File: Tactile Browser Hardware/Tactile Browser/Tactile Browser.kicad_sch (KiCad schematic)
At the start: 78 parts, among them SW1 SW_Push, SW10 SW_Push, SW11 SW_Push, SW12 SW_Push, SW13 SW_Push, SW14 SW_Push, SW15 SW_Push, SW16 SW_Push, SW17 SW_Push, SW18 SW_Push, SW19 SW_Push, SW2 SW_Push, SW20 SW_Push, SW3 SW_Push, SW4 SW_Push, SW5 SW_Push, SW6 SW_Push, SW7 SW_Push, SW8 SW_Push, SW9 SW_Push

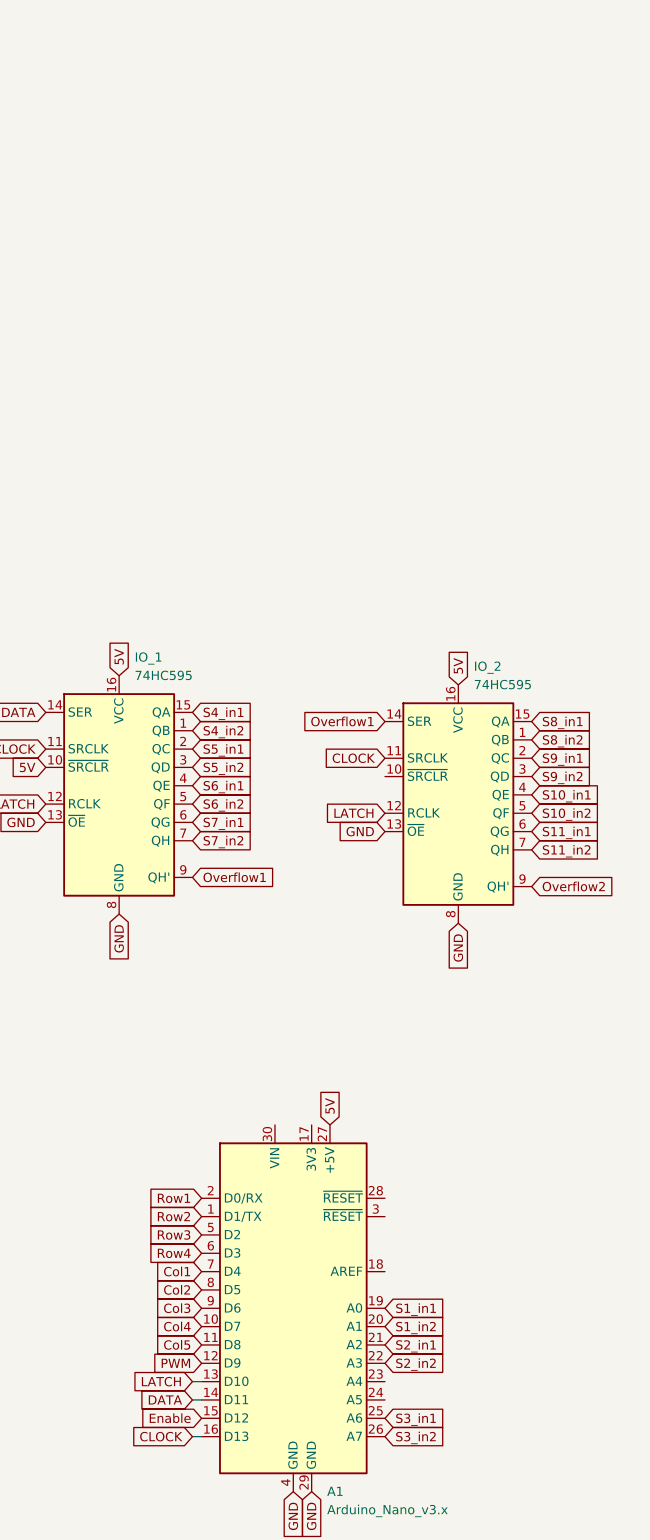
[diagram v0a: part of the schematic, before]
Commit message: I2C
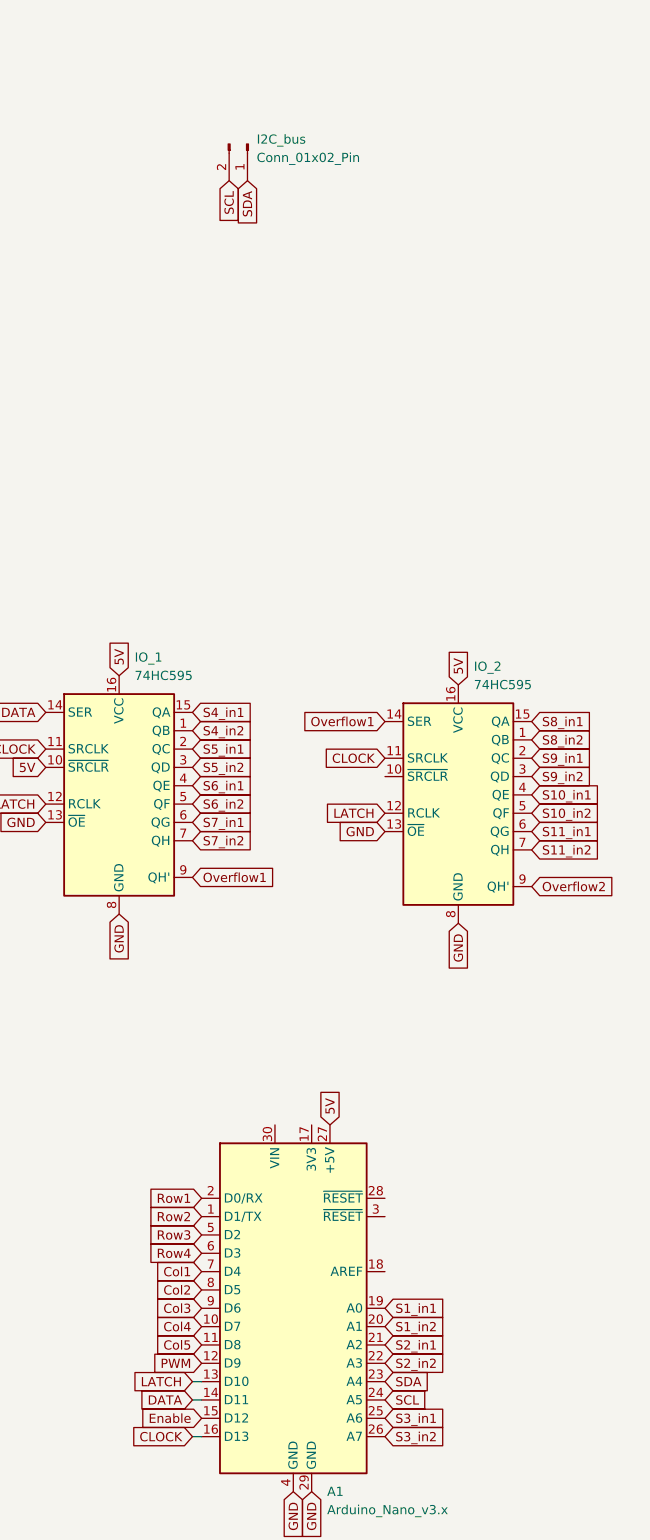
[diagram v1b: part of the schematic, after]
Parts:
- added I2C_bus: Conn_01x02_Pin, symbol Connector:Conn_01x02_Pin
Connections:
- net SDA: now reaches A1.23 (A4)
- net SDA: now also I2C_bus.1 (Pin_1)
- net SCL: now reaches A1.24 (A5)
- net SCL: now also I2C_bus.2 (Pin_2)
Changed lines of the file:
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@@
 		)
 	)
+	(global_label "SCL"
+		(shape input)
+		(at 254 71.12 270)
+		(fields_autoplaced yes)
+		(effects
+			(font
+				(size 1.27 1.27)
+			)
+			(justify right)
+		)
+		(property "Intersheetrefs" "${INTERSHEET_REFS}"
+			(at 254 77.6128 90)
+			(effects
+				(font
+					(size 1.27 1.27)
+				)
+				(justify right)
+				(hide yes)
+			)
+		)
+	)
 	(global_label "S2_in1"
 		(shape input)
@@
 		)
 	)
+	(global_label "SDA"
+		(shape input)
+		(at 256.54 71.12 270)
+		(fields_autoplaced yes)
+		(effects
+			(font
+				(size 1.27 1.27)
+			)
+			(justify right)
+		)
+		(property "Intersheetrefs" "${INTERSHEET_REFS}"
+			(at 256.54 77.6733 90)
+			(effects
+				(font
+					(size 1.27 1.27)
+				)
+				(justify right)
+				(hide yes)
+			)
+		)
+	)
 	(global_label "12V"
 		(shape input)
@@
 		)
 	)
+	(global_label "SDA"
+		(shape input)
+		(at 275.59 237.49 0)
+		(fields_autoplaced yes)
+		(effects
+			(font
+				(size 1.27 1.27)
+			)
+			(justify left)
+		)
+		(property "Intersheetrefs" "${INTERSHEET_REFS}"
+			(at 282.1433 237.49 0)
+			(effects
+				(font
+					(size 1.27 1.27)
+				)
+				(justify left)
+				(hide yes)
+			)
+		)
+	)
 	(global_label "S18_out2"
 		(shape input)
@@
 		)
 	)
+	(global_label "SCL"
+		(shape input)
+		(at 275.59 240.03 0)
+		(fields_autoplaced yes)
+		(effects
+			(font
+				(size 1.27 1.27)
+			)
+			(justify left)
+		)
+		(property "Intersheetrefs" "${INTERSHEET_REFS}"
+			(at 282.0828 240.03 0)
+			(effects
+				(font
+					(size 1.27 1.27)
+				)
+				(justify left)
+				(hide yes)
+			)
+		)
+	)
 	(global_label "5V"
 		(shape input)
@@
 					(unit 1)
 				)
+			)
+		)
+	)
+	(symbol
+		(lib_id "Connector:Conn_01x02_Pin")
+		(at 256.54 66.04 270)
+		(unit 1)
+		(exclude_from_sim no)
+		(in_bom yes)
+		(on_board yes)
+		(dnp no)
+		(fields_autoplaced yes)
+		(property "Reference" "I2C_bus"
+			(at 257.81 65.4049 90)
+			(effects
+				(font
+					(size 1.27 1.27)
+				)
+				(justify left)
+			)
+		)
+		(property "Value" "Conn_01x02_Pin"
+			(at 257.81 67.9449 90)
+			(effects
+				(font
+					(size 1.27 1.27)
+				)
+				(justify left)
+			)
+		)
+		(property "Footprint" ""
+			(at 256.54 66.04 0)
+			(effects
+				(font
+					(size 1.27 1.27)
+				)
+				(hide yes)
+			)
+		)
+		(property "Datasheet" "~"
+			(at 256.54 66.04 0)
+			(effects
+				(font
+					(size 1.27 1.27)
+				)
+				(hide yes)
+			)
+		)
+		(property "Description" "Generic connector, single row, 01x02, script generated"
+			(at 256.54 66.04 0)
+			(effects
+				(font
+					(size 1.27 1.27)
+				)
+				(hide yes)
+			)
+		)
+		(pin "1"
+		)
+		(pin "2"
+		)
+		(instances
+			(project ""
+				(path "/2e399075-89ae-469c-893b-1284214b820d"
+					(reference "I2C_bus")
+					(unit 1)
+				)
